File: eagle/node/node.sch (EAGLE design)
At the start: 25 parts, among them IC2 7805TV, X1 MKDSN1,5/2-5,08, X2 MKDSN1,5/2-5,08, X3 MKDSN1,5/2-5,08, X4 MKDSN1,5/2-5,08

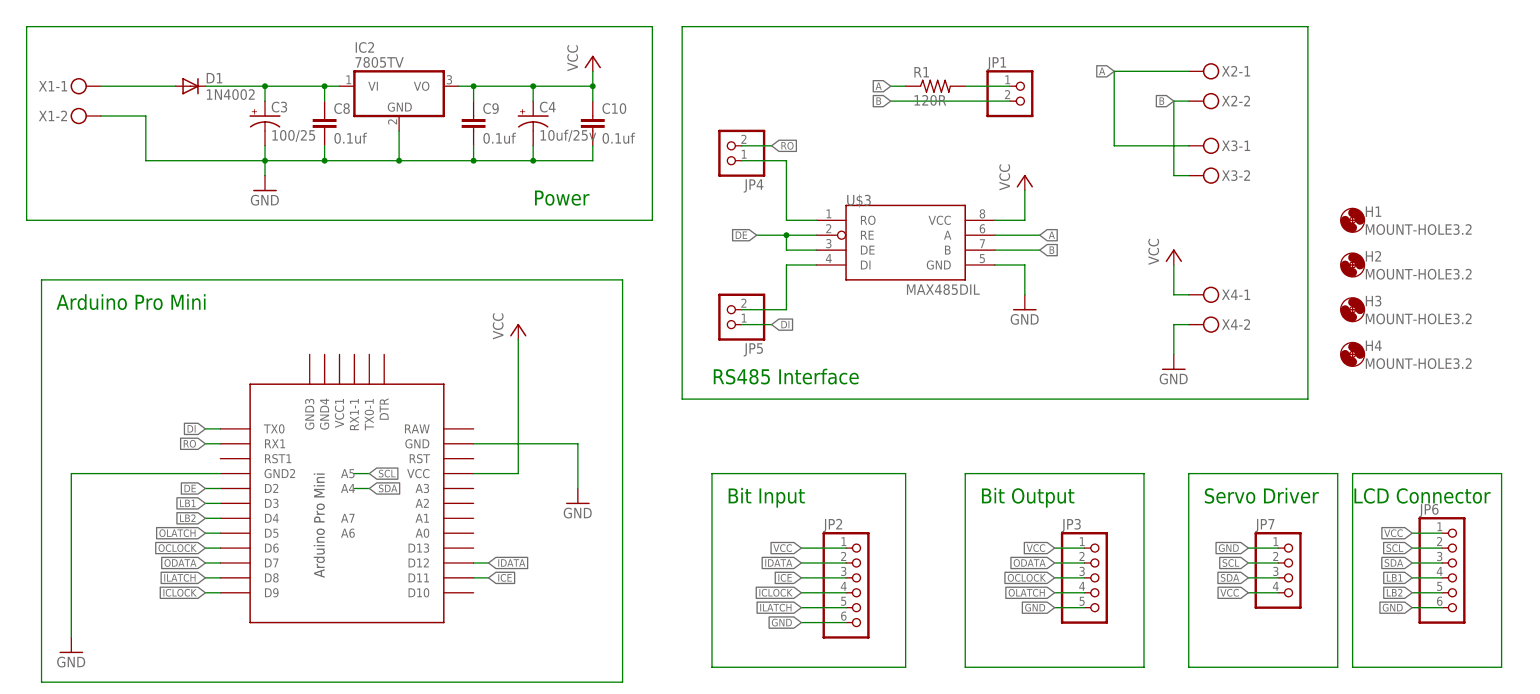
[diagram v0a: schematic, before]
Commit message: periodic checkin
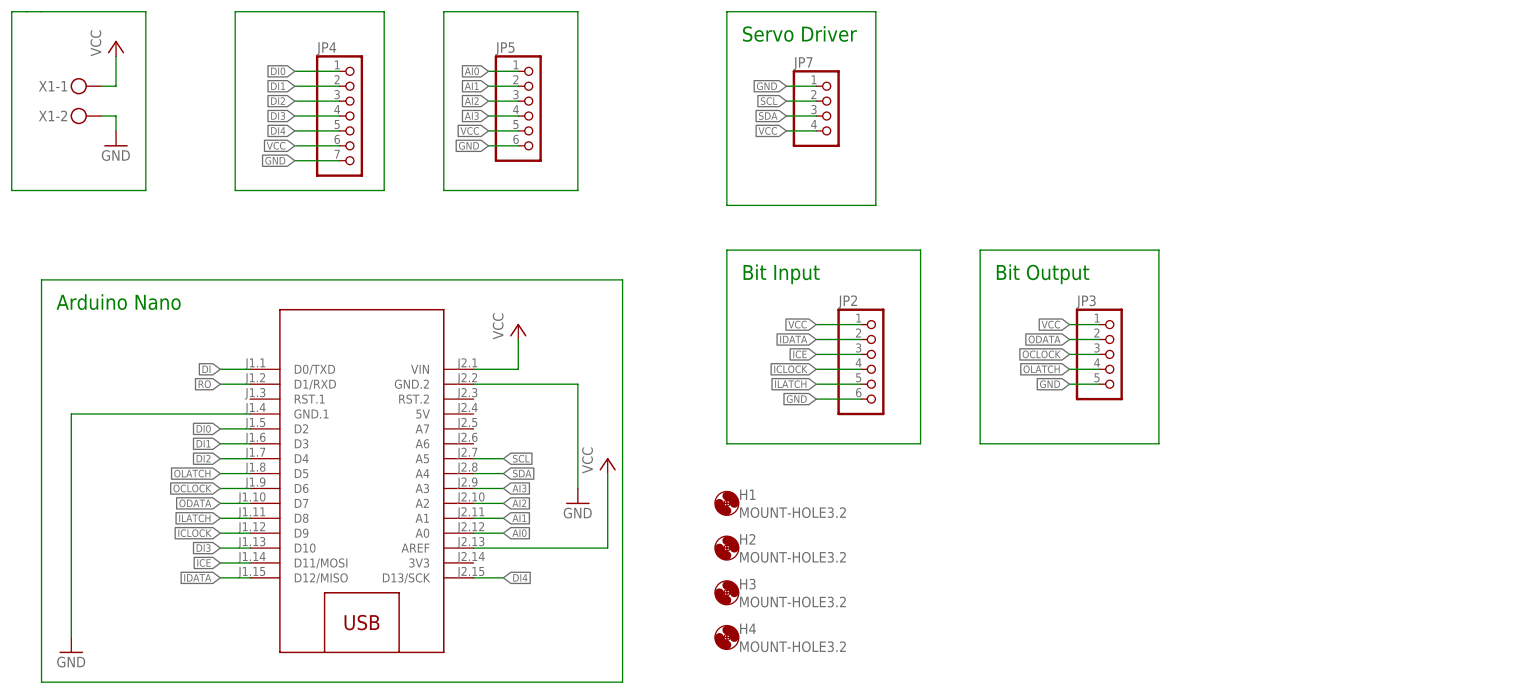
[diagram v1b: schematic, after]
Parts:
- removed C10, C8, C9: 0.1uf, resistor:C-EU025-025X050
- removed C3: 100/25, resistor:CPOL-USE2.5-7
- removed C4: 10uf/25v, resistor:CPOL-USE2-4
- removed D1: 1N4002, diode:1N4004
- removed IC2: 7805TV, linear:7805TV
- removed JP1: (no value), pinhead:PINHD-1X2
- removed JP6: (no value), pinhead:PINHD-1X6
- removed R1: 120R, resistor:R-US_0207/2V
- removed U$1: PRO-MINI-2, Arduino-clone:PRO-MINI-2
- removed U$3: MAX485DIL, SparkFun-DigitalIC:MAX485DIL
- removed X2, X3, X4: MKDSN1,5/2-5,08, con-phoenix-508:MKDSN1,5/2-5,08
- added M1: ARDUINO-NANO-3.0, diy-modules:ARDUINO-NANO-3.0
- JP4: device pinhead:PINHD-1X2 -> pinhead:PINHD-1X7
- JP5: device pinhead:PINHD-1X2 -> pinhead:PINHD-1X6
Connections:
- removed net A: R1.1, U$3.A, X2-1.KL, X3-1.KL
- removed net B: JP1.2, U$3.B, X2-2.KL, X3-2.KL
- removed net DE: U$1.D2, U$3.DE, U$3.RE
- removed net LB1: JP6.4, U$1.D3
- removed net LB2: JP6.5, U$1.D4
- removed net N$1: C3.+, C8.1, D1.C, IC2.VI
- removed net N$10: JP5.2, U$3.DI
- removed net N$11: JP4.1, U$3.RO
- removed net N$2: D1.A, X1-1.KL
- removed net N$3: JP1.1, R1.2
- new net AI0: JP5.1, M1.A0
- new net AI1: JP5.2, M1.A1
- new net AI2: JP5.3, M1.A2
- new net AI3: JP5.4, M1.A3
- new net DI0: JP4.1, M1.D2
- new net DI1: JP4.2, M1.D3
- new net DI2: JP4.3, M1.D4
- new net DI3: JP4.4, M1.D10
- new net DI4: JP4.5, M1.D13/SCK
- net DI: now also M1.D0/TXD; no longer JP5.1, U$1.TX0
- net GND: now also JP4.7, JP5.6, M1.GND.1, M1.GND.2; no longer C10.2, C3.-, C4.-, C8.2, C9.2, IC2.GND, JP6.6, U$1.GND, U$1.GND2, U$3.GND, X4-2.KL
- net ICE: now also M1.D11/MOSI; no longer U$1.D11
- net ICLOCK: now also M1.D9; no longer U$1.D9
- net IDATA: now also M1.D12/MISO; no longer U$1.D12
- net ILATCH: now also M1.D8; no longer U$1.D8
- net OCLOCK: now also M1.D6; no longer U$1.D6
- net ODATA: now also M1.D7; no longer U$1.D7
- net OLATCH: now also M1.D5; no longer U$1.D5
- net RO: now also M1.D1/RXD; no longer JP4.2, U$1.RX1
- net SCL: now also M1.A5; no longer JP6.2, U$1.A5
- net SDA: now also M1.A4; no longer JP6.3, U$1.A4
- net VCC: now also JP4.6, JP5.5, M1.AREF, M1.VIN, X1-1.KL; no longer C10.1, C4.+, C9.1, IC2.VO, JP6.1, U$1.VCC, U$3.VCC, X4-1.KL
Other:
- note added: "Arduino Nano"
- note removed: "Arduino Pro Mini"
- note removed: "LCD Connector"
- note removed: "Power"
- note removed: "RS485 Interface"
- moved on the sheet: H1, H2, H3, H4, JP2, JP3, JP7
